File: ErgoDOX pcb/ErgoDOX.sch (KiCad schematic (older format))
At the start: 64 parts, among them J1 USB, J2 3.5mm, J3 JMP, J4 JMP, SW0:10 SW0:3, SW0:11 SW0:2, SW0:12 SW0:1, SW0:7 SW0:6, SW0:8 SW0:5, SW0:9 SW0:4, SW1:10 SW1:3, SW1:11 SW1:2, SW1:12 SW1:1, SW1:13 SW1:0, SW1:9 SW1:4, SW2:10 SW2:3, SW2:11 SW2:2, SW2:12 SW2:1, SW2:13 SW2:0, SW2:7 SW2:6, SW2:8 SW2:5, SW2:9 SW2:4, SW3:10 SW3:3, SW3:11 SW3:2, SW3:12 SW3:1, SW3:13 SW3:0, SW3:8 SW3:5, SW3:9 SW3:4, SW4:10 SW4:3, SW4:11 SW4:2, SW4:12 SW4:1, SW4:13 SW4:0, SW4:7 SW4:6, SW4:8 SW4:5, SW4:9 SW4:4, SW5:10 SW5:3, SW5:11 SW5:2, SW5:12 SW5:1, SW5:13 SW5:0, SW5:7 SW5:6, SW5:8 SW5:5, SW5:9 SW5:4, U1 TEENSY2.0, U2 MCP23018

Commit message: added usb c to schema
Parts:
- removed J1: USB, symbol 6PIN
- added H1: D+, symbol Mechanical:MountingHole_Pad
- added H2: D-, symbol Mechanical:MountingHole_Pad
- added J1: USB, Connector_USB:USB_C_Receptacle_GCT_USB4085, symbol Connector:USB_C_Receptacle_USB2.0
- added R2, R3: 2.2kΩ, symbol component:RESISTOR
- D1:7, D1:8: symbol DIODE -> component:DIODE
- H99, S1, S2: symbol ANYTHING -> component:ANYTHING
- J2: symbol 6PIN -> component:6PIN
- J3, J4: symbol 3PIN -> component:3PIN
- JP1, JP2: symbol JUMPER -> component:JUMPER
- LED_A1, LED_B1, LED_C1: symbol LED -> component:LED
- R1, R2, RA1, RB1, RC1: symbol RESISTOR -> component:RESISTOR
- SW0:10, SW0:11, SW0:12, SW0:7, SW0:8, SW0:9, SW1:10, SW1:11, SW1:12, SW1:13, SW1:9, SW2:10, SW2:11, SW2:12, SW2:13, SW2:7, SW2:8, SW2:9, SW3:10, SW3:11, SW3:12, SW3:13, SW3:8, SW3:9, SW4:10, SW4:11, SW4:12, SW4:13, SW4:7, SW4:8, SW4:9, SW5:10, SW5:11, SW5:12, SW5:13, SW5:7, SW5:8, SW5:9: symbol SWITCH_DIODE -> component:SWITCH_DIODE
- SW_RST1, SX0:10, SX0:11, SX1:7, SX1:8: symbol SWITCH_PUSH -> component:SWITCH_PUSH
- U1: symbol TEENSY2.0 -> component:TEENSY2.0
- U2: symbol MCP23018 -> component:MCP23018
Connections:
- wire segments 172 -> 260
- no-connect marks 15 -> 17

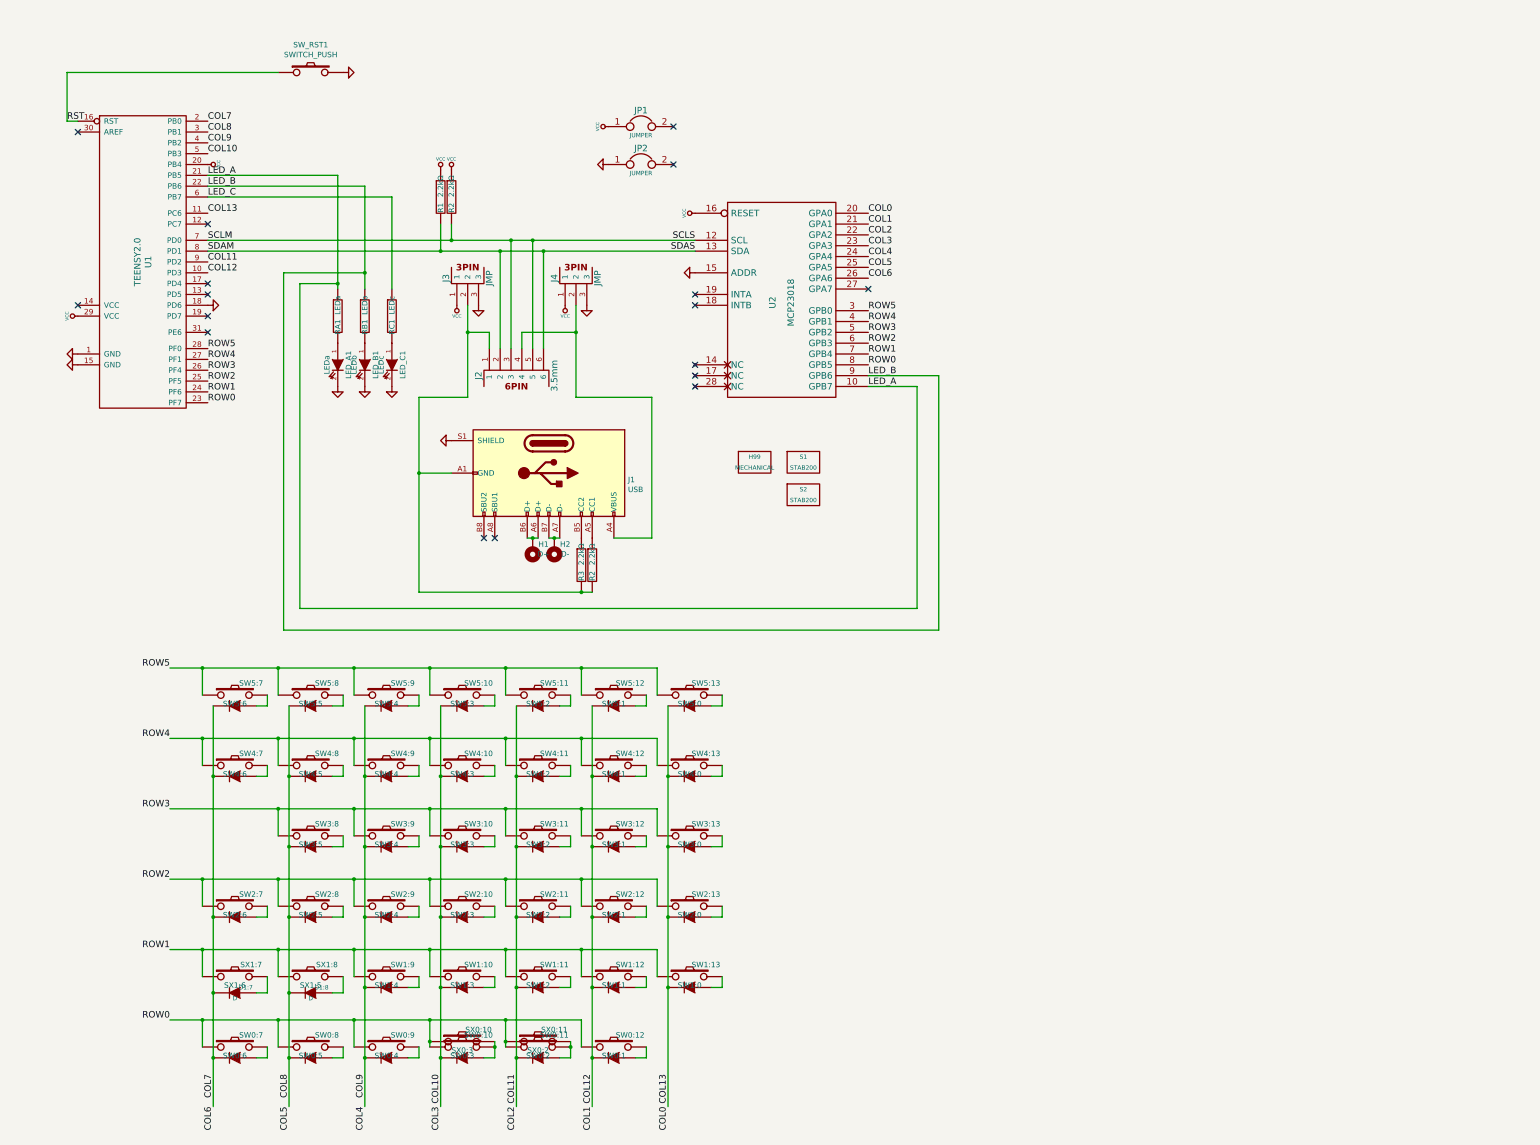
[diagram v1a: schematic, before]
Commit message: probably done
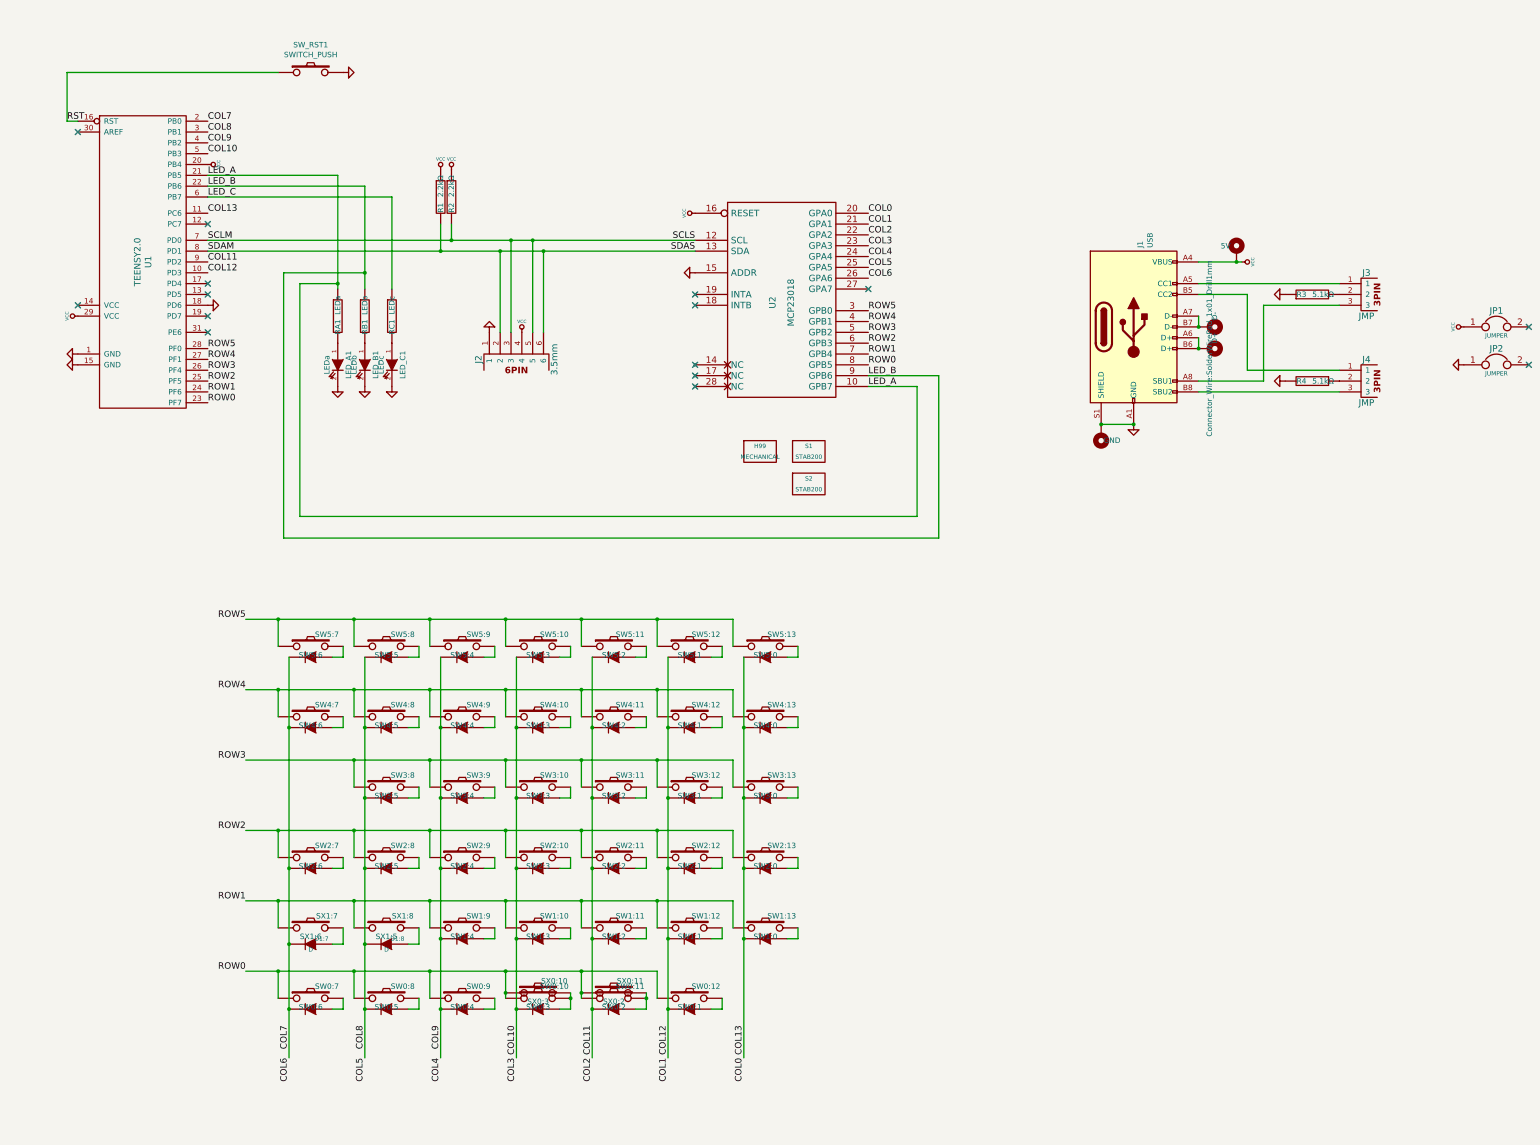
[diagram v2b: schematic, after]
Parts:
- added H3: 5V, Connector_Wire:SolderWirePad_1x01_Drill1mm, symbol Mechanical:MountingHole_Pad
- added H4: GND, Connector_Wire:SolderWirePad_1x01_Drill1mm, symbol Mechanical:MountingHole_Pad
- H1, H2: footprint (none) -> Connector_Wire:SolderWirePad_1x01_Drill1mm
- R3: renamed from R2; value 2.2kΩ -> 5.1kΩ; footprint (none) -> Resistor_THT:R_Axial_DIN0207_L6.3mm_D2.5mm_P10.16mm_Horizontal
- R4: renamed from R3; value 2.2kΩ -> 5.1kΩ; footprint (none) -> Resistor_THT:R_Axial_DIN0207_L6.3mm_D2.5mm_P10.16mm_Horizontal
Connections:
- net GND: now also J1.A1 (GND), J1.A12 (GND), J1.B1 (GND), J1.B12 (GND), J2.1, R3.1, R4.2, H4.1; no longer J3.3, J4.3
- net VCC: now also J1.A4 (VBUS), J1.A9 (VBUS), J1.B4 (VBUS), J1.B9 (VBUS), J2.4, H3.1; no longer J3.1, J4.1
- net at J1.A5 (CC1): now also J3.1; no longer R3.1
- net at J1.A8 (SBU1): now also J3.3
- net at J1.B5 (CC2): now also J4.1; no longer R4.1
- net at J1.B8 (SBU2): now also J4.3
- new net: J3.2, R3.2
- new net: J4.2, R4.1
- no-connect marks 17 -> 15
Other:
- moved on the sheet: D1:7, D1:8, H99, J1, J2, J3, J4, JP1, JP2, R3, R4, S1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
